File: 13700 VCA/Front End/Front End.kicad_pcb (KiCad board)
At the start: 2 copper layers, 80.9 x 104.5 mm, 32 parts, among them J1 AudioJack2_SwitchT, J10 Conn_01x19, J2 AudioJack2_SwitchT, J3 AudioJack2_SwitchT, J4 AudioJack2_SwitchT, J5 AudioJack2_SwitchT, J6 AudioJack2_SwitchT, J7 AudioJack2_SwitchT, J8 AudioJack2_SwitchT, J9 AudioJack2_SwitchT

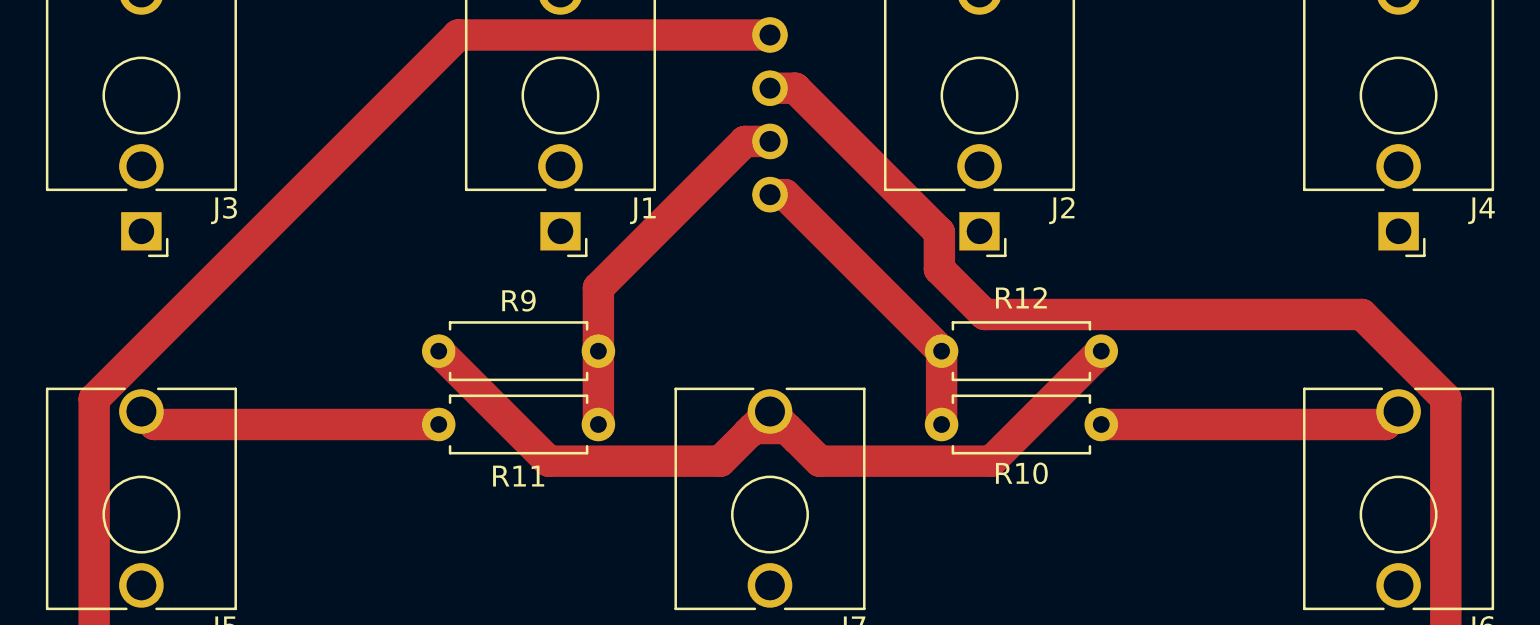
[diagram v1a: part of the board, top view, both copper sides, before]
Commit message: PCB fixes and cleanup
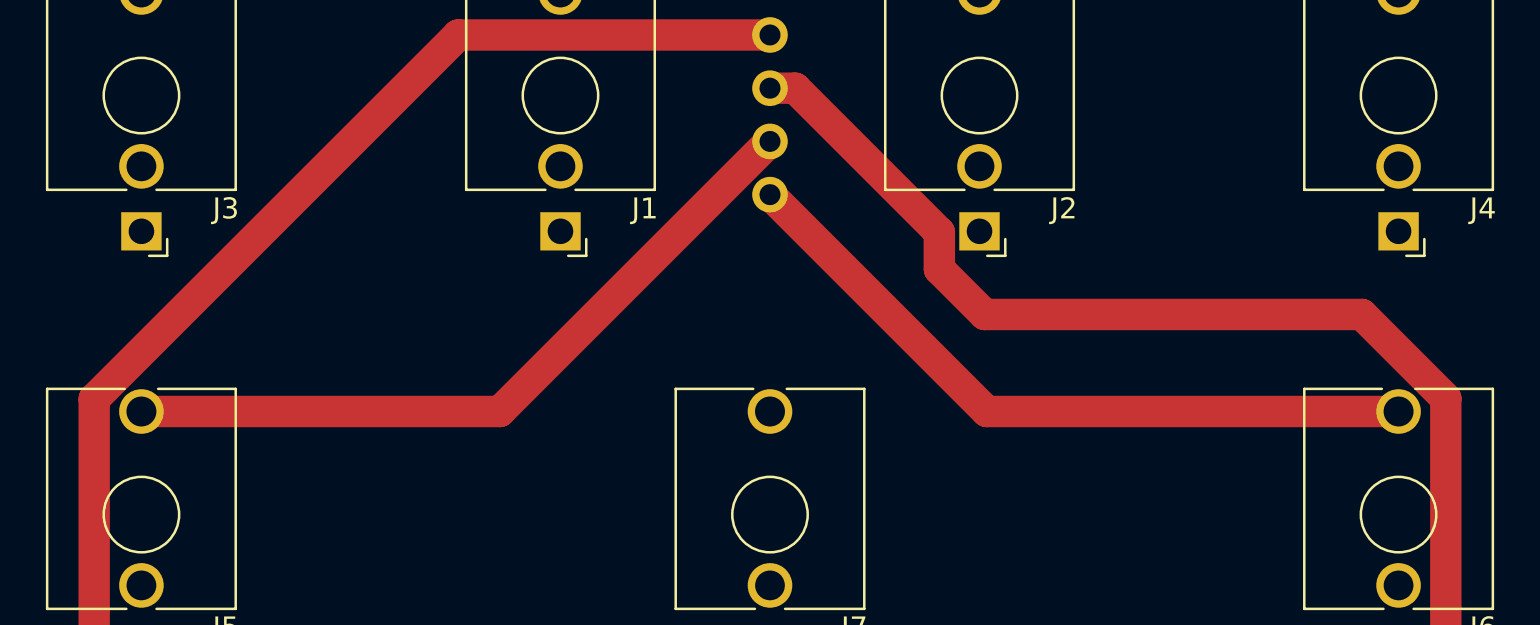
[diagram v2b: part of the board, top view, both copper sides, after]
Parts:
- removed R10, R11, R12, R9: 47k, Resistor_THT:R_Axial_DIN0207_L6.3mm_D2.5mm_P7.62mm_Horizontal
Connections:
- J5 pad T: Net-(J5-PadT) -> /IN_1
- J6 pad T: Net-(J6-PadT) -> /IN_2
- J7 pad T: Net-(J7-PadT) -> unconnected-(J7-PadT)
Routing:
- net Net-(J7-PadT): track 40.6 -> 0.00 mm
- net /IN_2: track 14.8 -> 34.3 mm
- net /IN_1: track 17.6 -> 35.3 mm
- net Net-(J6-PadT): track 14.4 -> 0.00 mm
- net Net-(J5-PadT): track 14.4 -> 0.00 mm
